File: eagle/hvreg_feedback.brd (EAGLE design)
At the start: 119.6 x 108.5 mm, 37 parts, among them K1 G5V-2, X4 BU-SMA-V

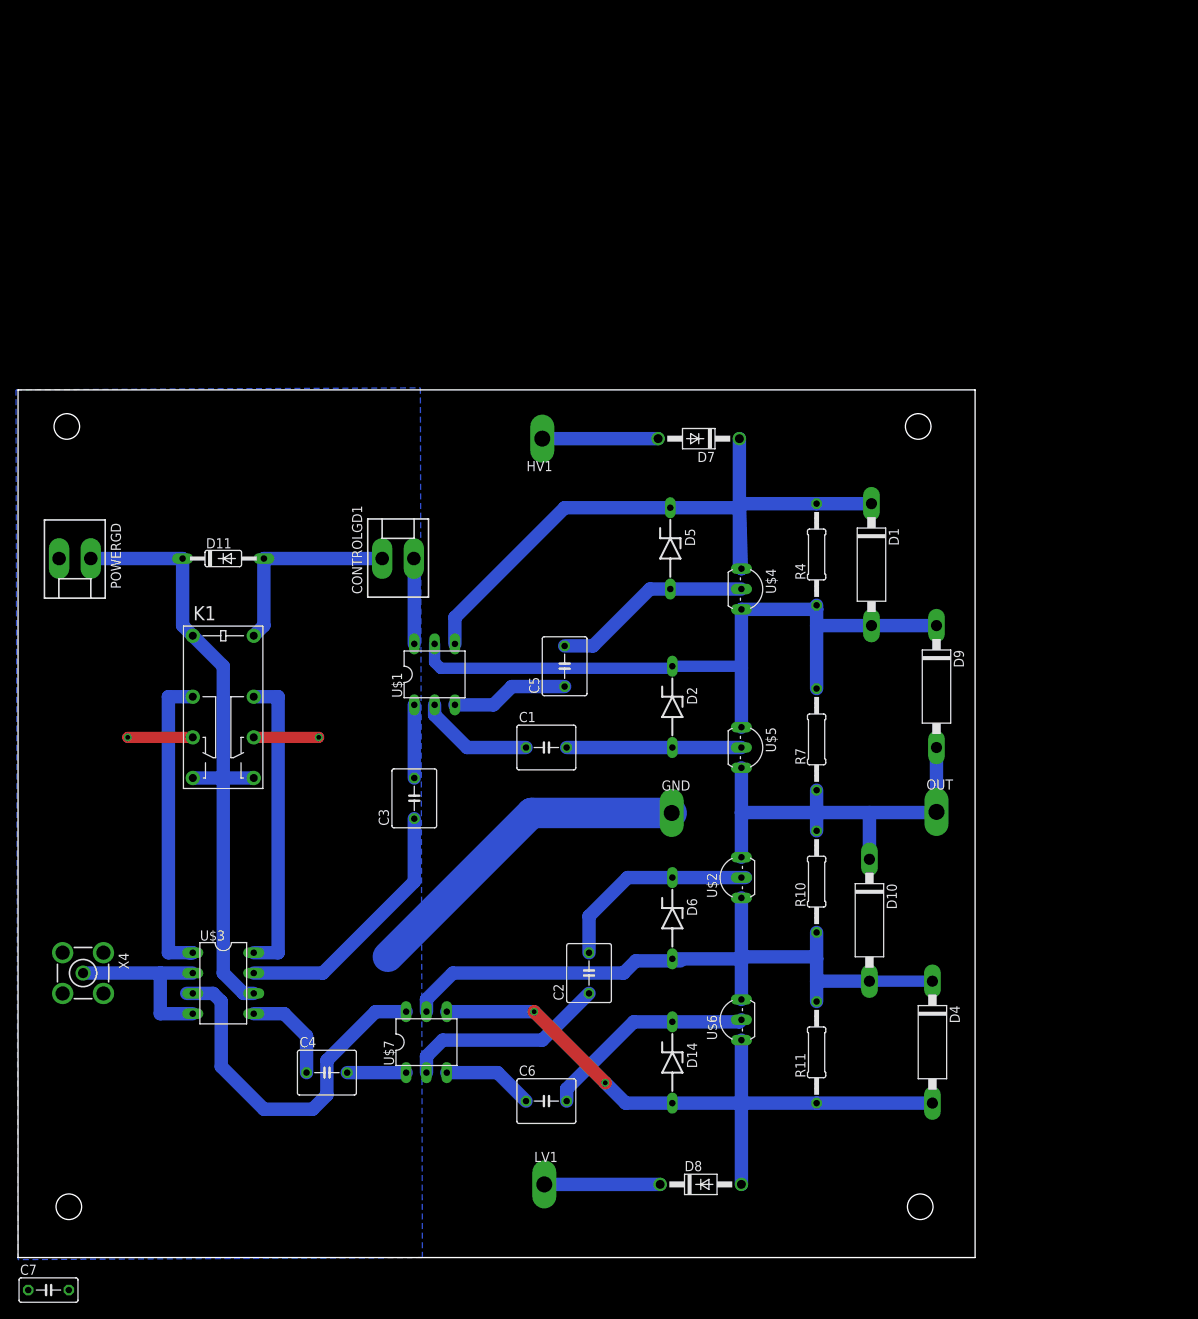
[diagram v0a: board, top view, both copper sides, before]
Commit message: feedback on hv rails
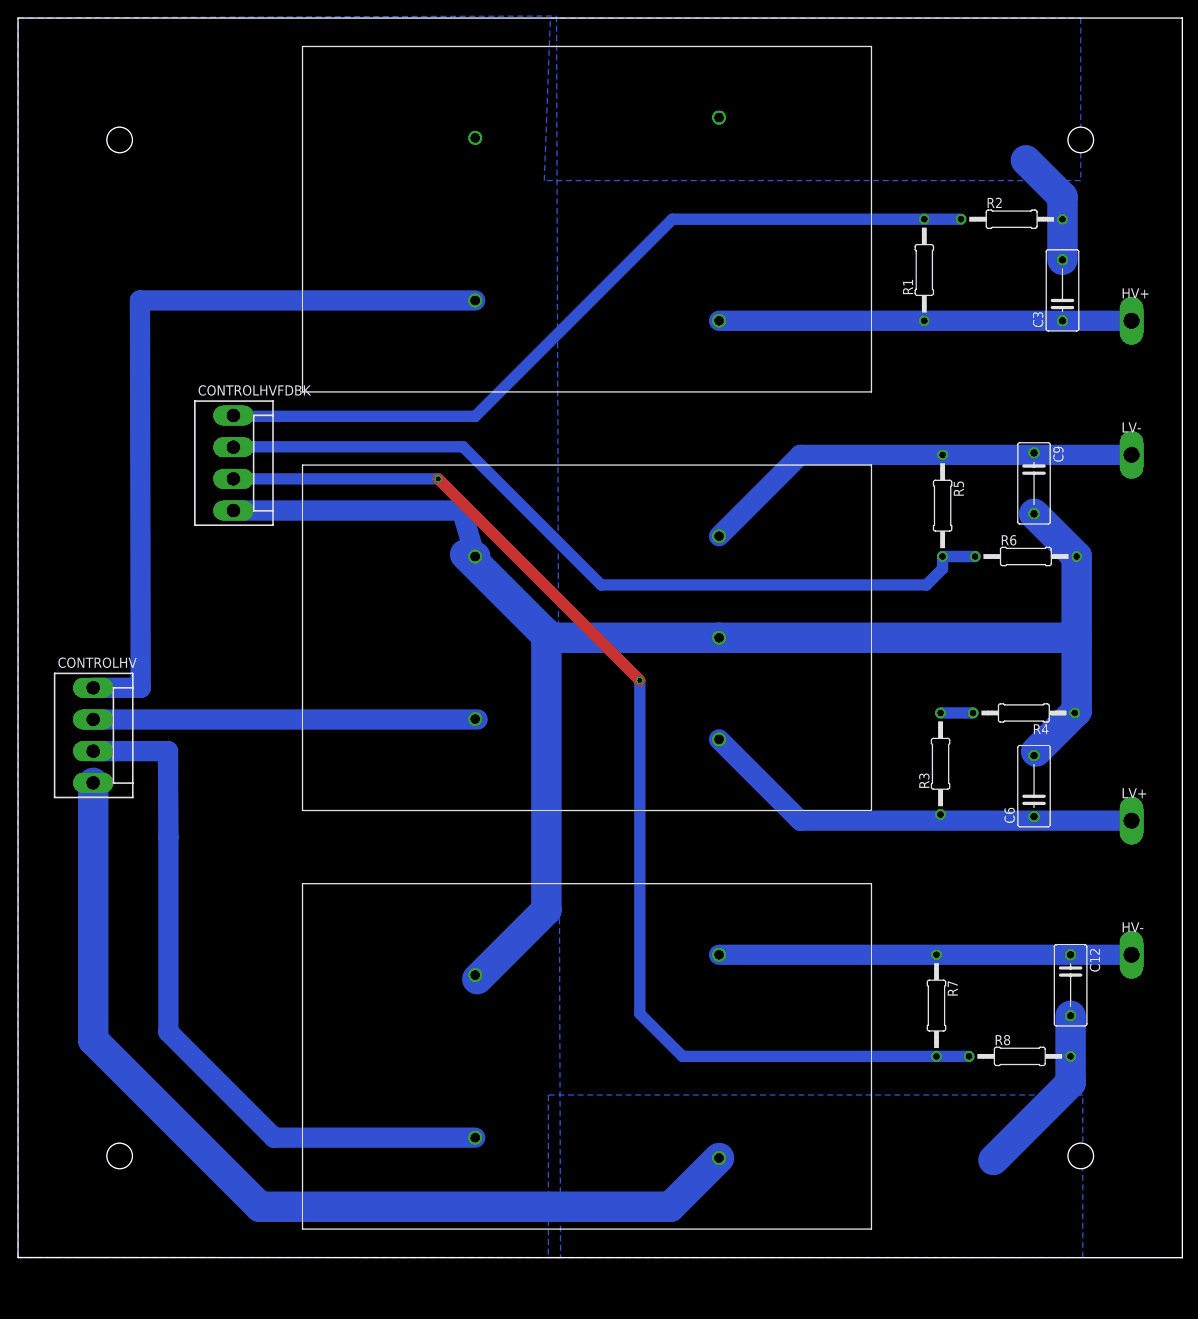
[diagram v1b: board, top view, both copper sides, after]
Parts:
- removed C1, C2, C4, C5: (no value), resistor:C050-055X075
- removed C7: (no value), rcl:C050-030X075
- removed CONTROLGD1, POWERGD: (no value), con-molex:KK-156-2
- removed D1, D10, D4, D9: P6KEXXA, diode:C1702-15
- removed D11: 1N4148DO35-10, diode:DO35-10
- removed D14, D2, D5, D6: 4742, diode:ZDIO-10
- removed D7, D8: 1N4004, diode:DO41-10
- removed GND, HV1, LV1, OUT: TPPAD1-20Y, testpad:P1-20Y
- removed K1: G5V-2, relay:G5V-2
- removed R10, R11: 1M, rcl:0207/12
- removed U$4, U$5: VP0550, transistor-fet:TO92-
- removed U$6: VN0550, transistor-fet:TO92-
- removed U$7: DA-2320, trafo:DIL06
- removed X4: BU-SMA-V, con-coax:BU-SMA-V
- added C12, C9: .01u, rcl:C075-042X103
- added CONTROLHV, CONTROLHVFDBK: (no value), con-molex:KK-156-4
- added HV+, HV-, LV+, LV-: TPPAD1-20Y, testpad:P1-20Y
- added R1, R2, R3, R5, R6, R8: (no value), resistor:0207/12
- C3, C6: value (none) -> .01u; device resistor:C050-055X075 -> rcl:C075-042X103
- R4, R7: value 1M -> (none); device rcl:0207/12 -> resistor:0207/12
- U$1: value DA-2320 -> EMCO-F104PIN; device trafo:DIL06 -> dc-dc-converter:EMCO-F
- U$2: value VN0550 -> EMCO-F20CT; device transistor-fet:TO92- -> dc-dc-converter:EMCO-F*CT
- U$3: value UCC27425 -> EMCO-F104PIN; device texas:DIL08 -> dc-dc-converter:EMCO-F
- moved C3 102.9 mm to (130.6, 120.9)
- moved C6 72.6 mm to (127.0, 58.9), turned to 90 degrees
- moved U$1 47.0 mm to (57.1, 119.6)
- moved U$2 38.7 mm to (57.1, 67.3), turned to 0 degrees
- moved U$3 36.9 mm to (57.1, 15.0), turned to 0 degrees
- moved R7 36.5 mm to (114.8, 31.5), turned to 270 degrees
- moved R4 32.6 mm to (125.7, 68.1), turned to 180 degrees
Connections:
- removed net +15V: C7.1, D11.C, K1.1, K1.8, K1.9, POWERGD.1, U$3.6
- removed net ENSW: CONTROLGD1.1, D11.A, K1.16
- removed net N$10: D8.C, LV1.TP
- removed net N$11: C1.2, D2.A, U$5.2
- removed net N$13: D10.A, D4.C, D6.A, R10.1, R11.2, U$2.3, U$6.1
- removed net N$14: K1.4, U$3.1
- removed net N$15: K1.13, U$3.8
- removed net N$16: C5.2, D5.A, U$4.2
- removed net N$17: D1.C, D5.C, D7.C, R4.2, U$1.4, U$4.3
- removed net N$18: D1.A, D2.C, D9.C, R4.1, R7.2, U$1.5, U$4.1, U$5.3
- removed net N$21: D10.C, D9.A, OUT.TP, R10.2, R7.1, U$2.1, U$5.1
- removed net N$22: C2.1, U$7.2
- removed net N$23: C6.1, U$7.3
- removed net N$25: C2.2, D6.C, U$2.2
- removed net N$27: C6.2, D14.C, U$6.2
- removed net N$29: D7.A, HV1.TP
- removed net N$30: D14.A, D4.A, D8.A, R11.1, U$6.3, U$7.4
- removed net N$9: U$7.5
- new net N$8: CONTROLHVFDBK.3, R7.2, R8.1
- new net VREG1: CONTROLHV.1, U$1.P$1
- new net VREG2: CONTROLHV.2, U$2.P$1
- new net VREG3: CONTROLHV.3, U$3.P$1
- net GND: now also C12.2, C3.2, C6.2, C9.2, CONTROLHV.4, CONTROLHVFDBK.4, R2.2, R4.1, R6.2, R8.2, U$1.P$2, U$1.P$4, U$2.P$2, U$2.P$5, U$3.P$2, U$3.P$3; no longer C7.2, CONTROLGD1.2, GND.TP, K1.11, K1.6, POWERGD.2, U$1.6, U$3.3, U$7.6, X4.2, X4.3, X4.4, X4.5
- net N$1: now also C3.1, HV+.TP, R1.1, U$1.P$3; no longer U$3.2, U$3.4, X4.1
- net N$2: now also C12.1, HV-.TP, R7.1, U$3.P$4; no longer C3.1, U$3.7
- net N$3: now also CONTROLHVFDBK.1, R1.2, R2.1; no longer C3.2, U$1.1
- net N$4: now also R3.2, R4.2; no longer C4.1, U$3.5
- net N$5: now also C6.1, LV+.TP, R3.1, U$2.P$3; no longer C1.1, U$1.2
- net N$6: now also C9.1, LV-.TP, R5.1, U$2.P$4; no longer C4.2, U$7.1
- net N$7: now also CONTROLHVFDBK.2, R5.2, R6.1; no longer C5.1, U$1.3
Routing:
- net GND: track 115.7 -> 367.4 mm, vias 2 -> 0
- net N$8: track 0.00 -> 146.3 mm, vias 0 -> 2
- net VREG1: track 0.00 -> 96.3 mm
- net N$3: track 9.14 -> 101.2 mm
- net N$18: track 90.7 -> 0.00 mm
- net VREG3: track 0.00 -> 88.3 mm
- net N$7: track 14.7 -> 102.3 mm
- net N$17: track 85.6 -> 0.00 mm
- net N$30: track 83.5 -> 0.00 mm, vias 2 -> 0
- net +15V: track 77.9 -> 0.00 mm
- net N$13: track 55.6 -> 0.00 mm
- net N$21: track 54.6 -> 0.00 mm
- net N$6: track 7.37 -> 55.6 mm
- net VREG2: track 0.00 -> 48.1 mm
- net N$5: track 14.4 -> 55.9 mm
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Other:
- board size 119.6 x 108.5 mm -> 145.5 x 155 mm
